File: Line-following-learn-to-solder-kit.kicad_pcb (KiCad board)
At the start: 2 copper layers, 73.9 x 104.6 mm, 25 parts, among them M1 DC TTMOTOR 3-6V, M2 DC TTMOTOR 3-6V, Q1 S8550, Q2 S8550

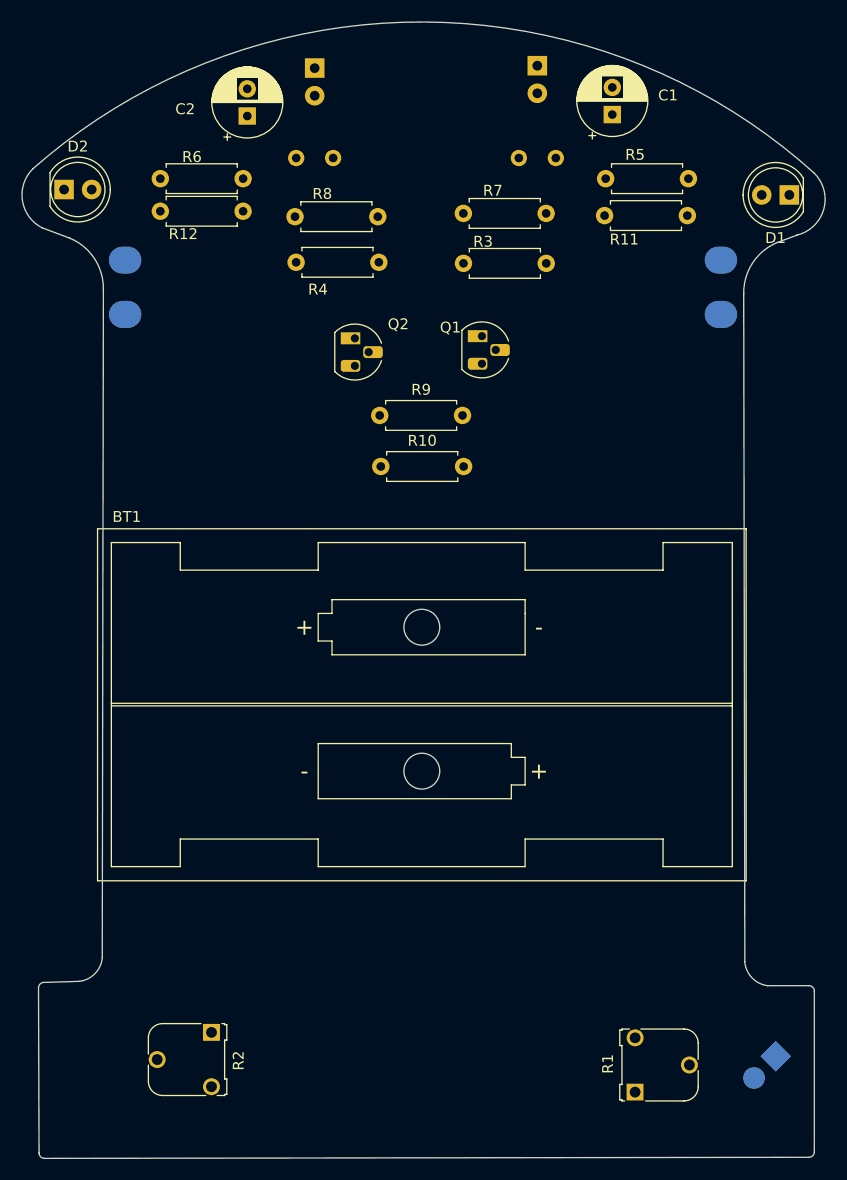
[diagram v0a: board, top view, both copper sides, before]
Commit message: v0.0 release. Still missing some 3d models, exact part number associations.
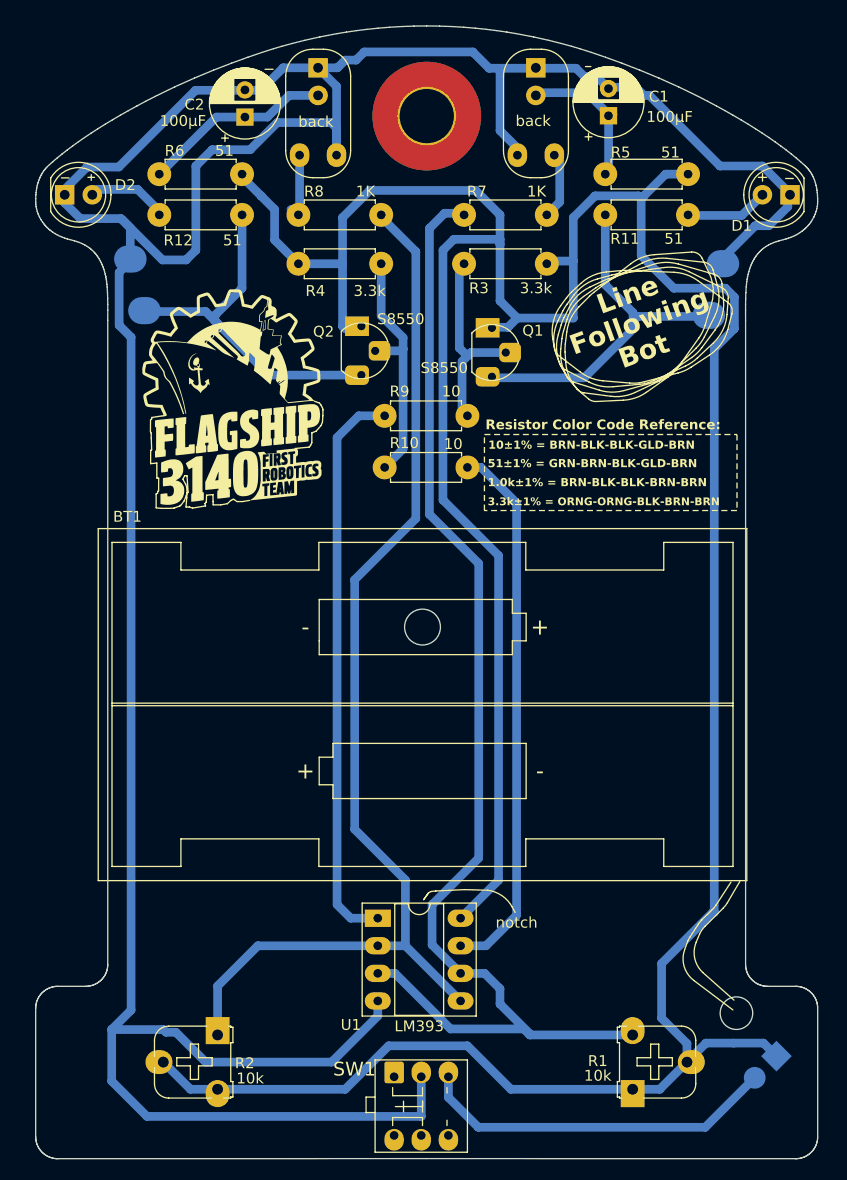
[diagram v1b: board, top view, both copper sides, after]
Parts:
- removed D3: LED2, LED_THT:LED_D5.0mm_Clear
- added D5: LED2, LED_THT:LED_D5.0mm_Clear, B.Cu at (80.8, 59.7)
- added G***: LOGO, LineFollowingRobotFootPrints:flagship logo, F.Cu at (73.0, 90.2)
- added H1: MountingHole for M5 skid foot, MountingHole:MountingHole_5mm_Pad_TopBottom, F.Cu at (90.8, 64.1)
- added H2: MountingHole for wires, LineFollowingRobotFootPrints:MountingHole_3mm, F.Cu at (119.3, 146.7)
- added SW1: SW_DPDT, LineFollowingRobotFootPrints:MHPS2283, F.Cu at (87.8, 152.6)
- added U1: LM393, Package_DIP:DIP-8_W7.62mm_Socket_LongPads, F.Cu at (86.3, 138.0)
- M2: footprint LineFollowingRobotFootPrints:TT-Motor -> LineFollowingRobotFootPrints:TT-Motor-mirrored
- Q1, Q2: footprint Package_TO_SOT_THT:TO-92_HandSolder -> LineFollowingRobotFootPrints:TO-92_HandSolder
- R1, R2: footprint Potentiometer_THT:Potentiometer_Runtron_RM-065_Vertical -> LineFollowingRobotFootPrints:Potentiometer_Runtron_RM-065_Vertical_hand_soldering
- R10, R11, R12, R3, R4, R5, R6, R7, R8, R9: footprint Resistor_THT:R_Axial_DIN0207_L6.3mm_D2.5mm_P7.62mm_Horizontal -> LineFollowingRobotFootPrints:R_Axial_DIN0207_L6.3mm_D2.5mm_P7.62mm_Horizontal_hand_soldering
- R13, R14: value LDR07 -> LDR; footprint OptoDevice:R_LDR_5.1x4.3mm_P3.4mm_Vertical -> LineFollowingRobotFootPrints:R_LDR_5.1x4.3mm_P3.4mm_Vertical_hand_soldering
- moved M2 58.1 mm to (110.6, 129.0), turned to 0 degrees
- moved M1 40.4 mm to (70.0, 128.6)
- moved R9 8.07 mm to (94.6, 91.7), turned to 180 degrees
- moved R10 7.97 mm to (94.6, 96.5), turned to 180 degrees
- moved R8 7.93 mm to (86.6, 73.2), turned to 180 degrees
- moved R12 7.53 mm to (73.8, 73.2), turned to 180 degrees
- moved R14 3.10 mm to (79.1, 67.7), turned to 0 degrees
- moved Q1 0.95 mm to (96.8, 84.6)
- moved Q2 0.61 mm to (84.8, 84.5)
- moved R2 0.61 mm to (71.6, 148.7)
- moved D2 0.49 mm to (57.5, 71.4)
- moved R6 0.43 mm to (66.2, 69.5)
- moved R5 0.42 mm to (107.3, 69.5)
- moved C1 0.37 mm to (107.5, 64.1)
- moved R1 0.35 mm to (109.8, 153.7)
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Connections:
- C2 pad 1: Net-(D3-A) -> Net-(D5-A)
- M1 pad 1: Net-(M1-+) -> Net-(D1-K)
- M1 pad 2: Net-(D1-K) -> Net-(M1--)
- M2 pad 1: Net-(M2-+) -> Net-(D1-K)
- M2 pad 2: Net-(D1-K) -> Net-(M2--)
- Q1 pad 3: Net-(M1-+) -> Net-(M2--)
- Q2 pad 3: Net-(M2-+) -> Net-(M1--)
- R11 pad 1: Net-(M1-+) -> Net-(M2--)
- R12 pad 1: Net-(M2-+) -> Net-(M1--)
- R2 pad 1: Net-(BT1-+) -> Net-(U1A--)
- R2 pad 3: Net-(U1A--) -> Net-(BT1-+)
- R4 pad 1: Net-(Q2-B) -> Net-(BT1-+)
- R4 pad 2: Net-(BT1-+) -> Net-(Q2-B)
- R5 pad 1: Net-(BT1-+) -> Net-(D4-A)
- R5 pad 2: Net-(D4-A) -> Net-(BT1-+)
- R6 pad 1: Net-(BT1-+) -> Net-(D5-A)
- R6 pad 2: Net-(D3-A) -> Net-(BT1-+)
- R9 pad 1: Net-(R9-Pad1) -> Net-(Q1-B)
- R9 pad 2: Net-(Q1-B) -> Net-(R9-Pad2)
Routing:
- net Net-(BT1-+): track 0.00 -> 307.9 mm
- net Net-(D1-K): track 0.00 -> 290.4 mm
- net Net-(U1A-+): track 0.00 -> 112.5 mm
- net Net-(U1A--): track 0.00 -> 103.1 mm
- net Net-(R9-Pad2): track 0.00 -> 52.5 mm
- net Net-(R10-Pad1): track 0.00 -> 50.3 mm
- net Net-(M2--): track 0.00 -> 33.6 mm
- net Net-(M1--): track 0.00 -> 33.1 mm
- net Net-(BT1--): track 0.00 -> 33.1 mm
- net Net-(Q2-B): track 0.00 -> 23.1 mm
- net Net-(Q1-B): track 0.00 -> 18.8 mm
- net Net-(D5-A): track 0.00 -> 17.6 mm
- net Net-(D4-A): track 0.00 -> 13.8 mm
- net Net-(D1-A): track 0.00 -> 7.64 mm
- net Net-(D2-A): track 0.00 -> 7.20 mm
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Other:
- board size 73.9 x 104.6 mm -> 72 x 104.3 mm
- board text added: "1.0k±1% = BRN-BLK-BLK-BRN-BRN"
- board text added: "10±1% = BRN-BLK-BLK-GLD-BRN"
- board text added: "3.3k±1% = ORNG-ORNG-BLK-BRN-BRN"
- board text added: "51±1% = GRN-BRN-BLK-GLD-BRN"
- board text added: "Bot"
- board text added: "Following"
- board text added: "Line"
- board text added: "Resistor Color Code Reference:"
- board text added: "back"
- board text added: "notch"
